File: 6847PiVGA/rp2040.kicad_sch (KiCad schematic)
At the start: 27 parts, among them J3 Program, U10 RP2040, U8 AMS1117-3.3, U9 W25Q128JVS, Y2 12MHz

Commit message: complete routing
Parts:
- C18, C21: footprint Capacitor_SMD:C_0603_1608Metric -> Capacitor_SMD:C_0805_2012Metric_Pad1.18x1.45mm_HandSolder
- C19, C20, C26, C27, C28, C29, C30, C31, C32, C33: footprint Capacitor_SMD:C_0402_1005Metric -> Capacitor_SMD:C_0603_1608Metric_Pad1.08x0.95mm_HandSolder
- C22: footprint Capacitor_SMD:C_0402_1005Metric -> Capacitor_SMD:C_0805_2012Metric_Pad1.18x1.45mm_HandSolder
- D2: footprint Diode_SMD:D_0603_1608Metric -> Diode_SMD:D_0805_2012Metric_Pad1.15x1.40mm_HandSolder
- R25: footprint Resistor_SMD:R_0603_1608Metric -> Resistor_SMD:R_0805_2012Metric_Pad1.20x1.40mm_HandSolder
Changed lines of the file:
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@@
 			)
 		)
-		(property "Footprint" "Capacitor_SMD:C_0603_1608Metric"
+		(property "Footprint" "Capacitor_SMD:C_0805_2012Metric_Pad1.18x1.45mm_HandSolder"
 			(at 43.18 57.15 0)
 			(effects
@@
 			)
 		)
-		(property "Footprint" "Capacitor_SMD:C_0603_1608Metric"
+		(property "Footprint" "Capacitor_SMD:C_0805_2012Metric_Pad1.18x1.45mm_HandSolder"
 			(at 25.4 57.15 0)
 			(effects
@@
 			)
 		)
-		(property "Footprint" "Capacitor_SMD:C_0402_1005Metric"
+		(property "Footprint" "Capacitor_SMD:C_0603_1608Metric_Pad1.08x0.95mm_HandSolder"
 			(at 217.17 40.64 0)
 			(effects
@@
 			)
 		)
-		(property "Footprint" "Resistor_SMD:R_0603_1608Metric"
+		(property "Footprint" "Resistor_SMD:R_0805_2012Metric_Pad1.20x1.40mm_HandSolder"
 			(at 69.85 114.3 0)
 			(effects
@@
 			)
 		)
-		(property "Footprint" "Diode_SMD:D_0603_1608Metric"
+		(property "Footprint" "Diode_SMD:D_0805_2012Metric_Pad1.15x1.40mm_HandSolder"
 			(at 76.2 114.3 0)
 			(effects
@@
 			)
 		)
-		(property "Footprint" "Capacitor_SMD:C_0402_1005Metric"
+		(property "Footprint" "Capacitor_SMD:C_0603_1608Metric_Pad1.08x0.95mm_HandSolder"
 			(at 207.01 40.64 0)
 			(effects
@@
 			)
 		)
-		(property "Footprint" "Capacitor_SMD:C_0402_1005Metric"
+		(property "Footprint" "Capacitor_SMD:C_0603_1608Metric_Pad1.08x0.95mm_HandSolder"
 			(at 176.53 40.64 0)
 			(effects
@@
 			)
 		)
-		(property "Footprint" "Capacitor_SMD:C_0402_1005Metric"
+		(property "Footprint" "Capacitor_SMD:C_0603_1608Metric_Pad1.08x0.95mm_HandSolder"
 			(at 237.49 40.64 0)
 			(effects
@@
 			)
 		)
-		(property "Footprint" "Capacitor_SMD:C_0402_1005Metric"
+		(property "Footprint" "Capacitor_SMD:C_0805_2012Metric_Pad1.18x1.45mm_HandSolder"
 			(at 86.36 157.7848 0)
 			(effects
@@
 			)
 		)
-		(property "Footprint" "Capacitor_SMD:C_0402_1005Metric"
+		(property "Footprint" "Capacitor_SMD:C_0603_1608Metric_Pad1.08x0.95mm_HandSolder"
 			(at 26.67 88.9 0)
 			(effects
@@
 			)
 		)
-		(property "Footprint" "Capacitor_SMD:C_0402_1005Metric"
+		(property "Footprint" "Capacitor_SMD:C_0603_1608Metric_Pad1.08x0.95mm_HandSolder"
 			(at 41.91 88.9 0)
 			(effects
@@
 			)
 		)
-		(property "Footprint" "Capacitor_SMD:C_0402_1005Metric"
+		(property "Footprint" "Capacitor_SMD:C_0603_1608Metric_Pad1.08x0.95mm_HandSolder"
 			(at 227.33 40.64 0)
 			(effects
@@
 			)
 		)
-		(property "Footprint" "Capacitor_SMD:C_0402_1005Metric"
+		(property "Footprint" "Capacitor_SMD:C_0603_1608Metric_Pad1.08x0.95mm_HandSolder"
 			(at 175.26 53.34 0)
 			(effects
@@
 			)
 		)
-		(property "Footprint" "Capacitor_SMD:C_0402_1005Metric"
+		(property "Footprint" "Capacitor_SMD:C_0603_1608Metric_Pad1.08x0.95mm_HandSolder"
 			(at 196.85 40.64 0)
 			(effects
@@
 			)
 		)
-		(property "Footprint" "Capacitor_SMD:C_0402_1005Metric"
+		(property "Footprint" "Capacitor_SMD:C_0603_1608Metric_Pad1.08x0.95mm_HandSolder"
 			(at 186.69 40.64 0)
 			(effects

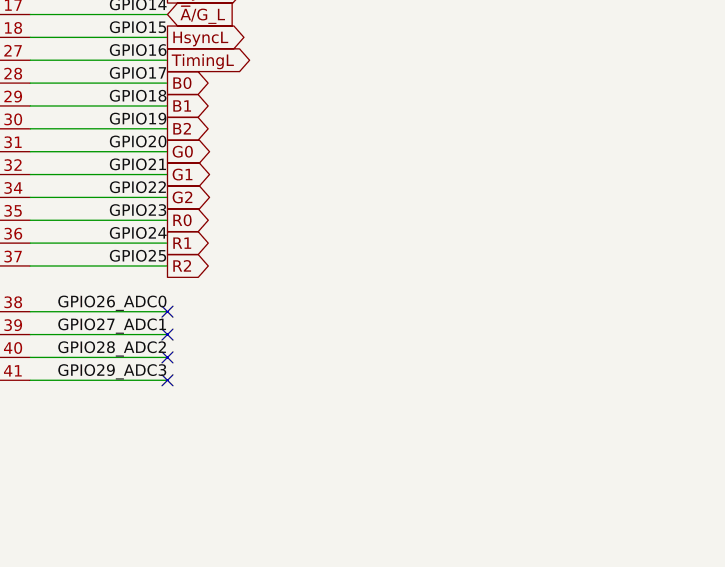
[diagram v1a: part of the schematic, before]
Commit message: refine pcb routing
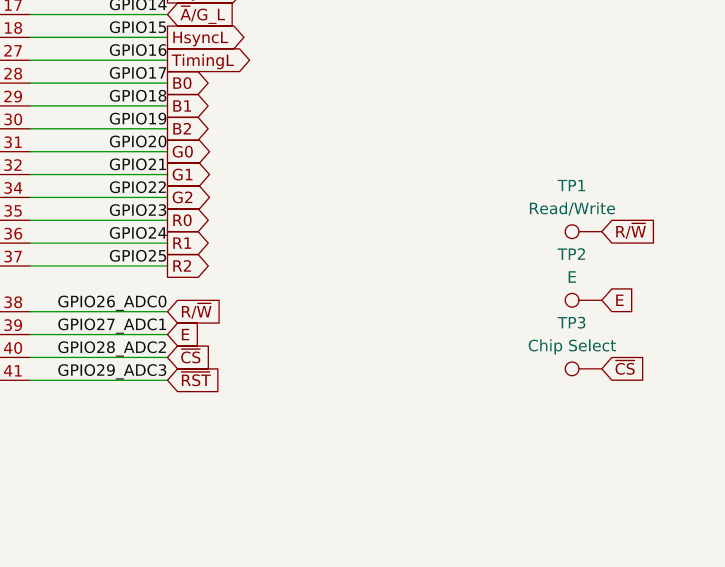
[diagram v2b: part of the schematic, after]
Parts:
- added TP1: Read/Write, TestPoint:TestPoint_Loop_D1.80mm_Drill1.0mm_Beaded, symbol Connector:TestPoint
- added TP2: E, TestPoint:TestPoint_Loop_D1.80mm_Drill1.0mm_Beaded, symbol Connector:TestPoint
- added TP3: Chip Select, TestPoint:TestPoint_Loop_D1.80mm_Drill1.0mm_Beaded, symbol Connector:TestPoint
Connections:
- net GPIO26_ADC0 renamed R/~{W}
- net R/~{W}: now also TP1.1
- net GPIO27_ADC1 renamed E
- net E: now also TP2.1
- net GPIO28_ADC2 renamed ~{CS}
- net ~{CS}: now also TP3.1
- net GPIO29_ADC3 renamed ~{RST}
- no-connect marks 4 -> 0
